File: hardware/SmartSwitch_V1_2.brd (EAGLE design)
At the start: 49 x 49 mm, 47 parts, among them K1 FTR-LYC5, K2 FTR-LYC5, U2 AMS1117-3.3

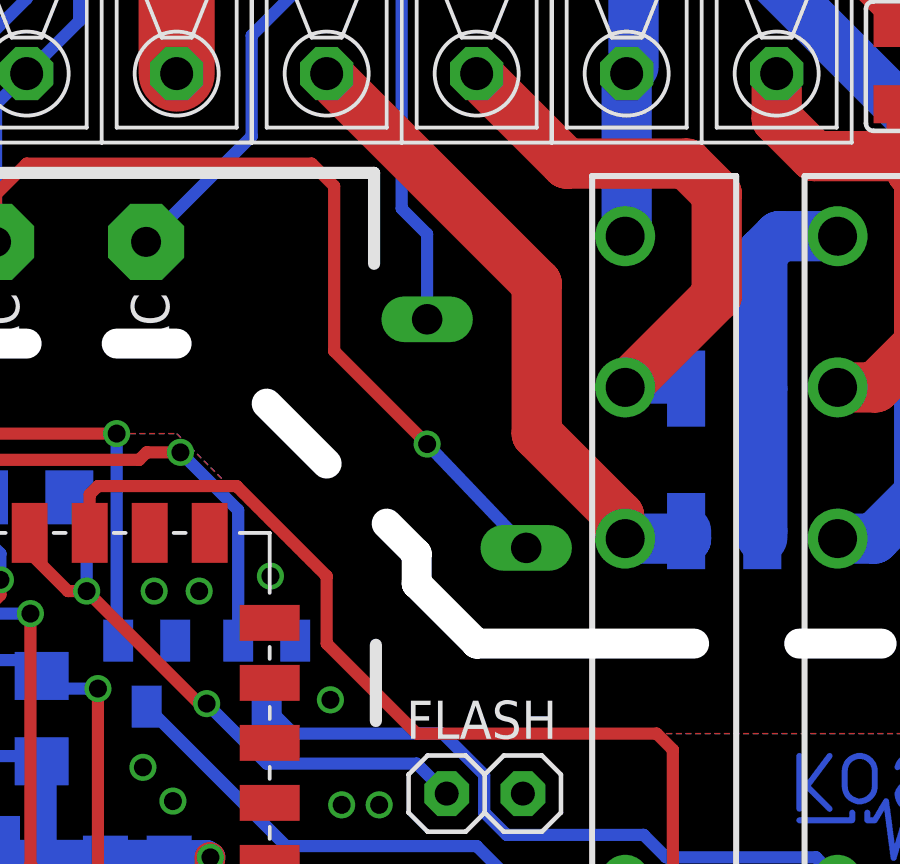
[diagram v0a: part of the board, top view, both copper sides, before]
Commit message: Add files via upload
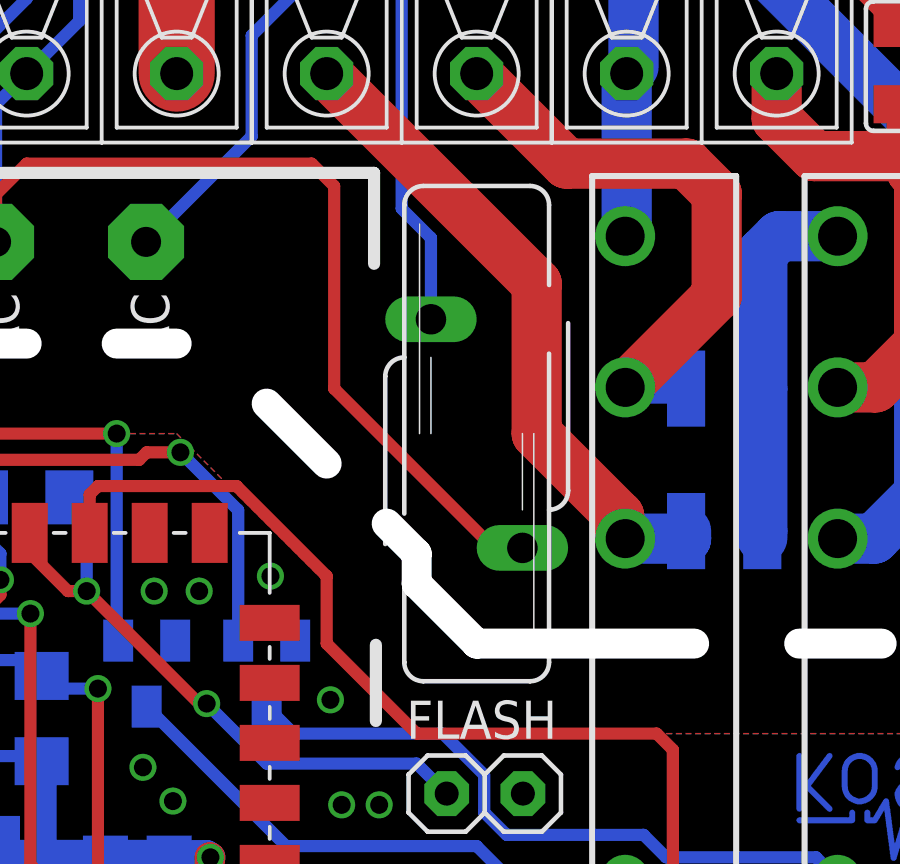
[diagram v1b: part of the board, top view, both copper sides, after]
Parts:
- R7: value S14K275 -> S14K275GESPIEGELT; device varistor:S14K275 -> varistor:S14K275_
- flipped R7 to the top
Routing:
- net HV.N: track 49.5 -> 50.1 mm, vias 1 -> 0
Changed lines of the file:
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@@
 <layer number="23" name="tOrigins" color="15" fill="1" visible="yes" active="yes"/>
 <layer number="24" name="bOrigins" color="15" fill="1" visible="yes" active="yes"/>
-<layer number="25" name="tNames" color="7" fill="1" visible="yes" active="yes"/>
-<layer number="26" name="bNames" color="7" fill="1" visible="yes" active="yes"/>
-<layer number="27" name="tValues" color="7" fill="1" visible="yes" active="yes"/>
-<layer number="28" name="bValues" color="7" fill="1" visible="yes" active="yes"/>
+<layer number="25" name="tNames" color="7" fill="1" visible="no" active="yes"/>
+<layer number="26" name="bNames" color="7" fill="1" visible="no" active="yes"/>
+<layer number="27" name="tValues" color="7" fill="1" visible="no" active="yes"/>
+<layer number="28" name="bValues" color="7" fill="1" visible="no" active="yes"/>
 <layer number="29" name="tStop" color="7" fill="3" visible="no" active="yes"/>
 <layer number="30" name="bStop" color="7" fill="6" visible="no" active="yes"/>
@@
 <attribute name="VALUE" x="17.54" y="19.27" size="1.27" layer="28" rot="MR270"/>
 </element>
-<element name="R7" library="varistor" package="S14K275" value="S14K275" x="32" y="26.5" smashed="yes" rot="MR0">
-<attribute name="VALUE" x="35.429" y="26.119" size="1.27" layer="28" ratio="10" rot="MR90"/>
+<element name="R7" library="varistor" package="S14K275_" value="S14K275GESPIEGELT" x="32" y="26.5" smashed="yes">
+<attribute name="VALUE" x="28.571" y="26.119" size="1.27" layer="27" ratio="10" rot="R90"/>
 </element>
 <element name="F1" library="fuse" package="SMD_FUSE_HOLDER" value="0,4A" x="25" y="43.5" smashed="yes" rot="MR180"/>
@@
 <wire x1="17" y1="35.5" x2="26.5" y2="35.5" width="0.4064" layer="1"/>
 <wire x1="26.5" y1="35.5" x2="27.25" y2="34.75" width="0.4064" layer="1"/>
-<wire x1="27.25" y1="34.75" x2="27.25" y2="29.25" width="0.4064" layer="1"/>
-<wire x1="27.25" y1="29.25" x2="30.349" y2="26.151" width="0.4064" layer="1"/>
-<wire x1="30.349" y1="26.151" x2="33.651" y2="22.69" width="0.4064" layer="16"/>
+<wire x1="27.25" y1="34.75" x2="27.25" y2="28" width="0.4064" layer="1"/>
 <contactref element="R2" pad="1"/>
 <contactref element="R4" pad="1"/>
@@
 <wire x1="18.75" y1="46.25" x2="18.75" y2="40.25" width="0.4064" layer="16"/>
 <wire x1="18.75" y1="40.25" x2="17" y2="38.5" width="0.4064" layer="16"/>
-<via x="30.349" y="26.151" extent="1-16" drill="0.6" shape="octagon"/>
 <wire x1="12.422" y1="46" x2="14.25" y2="46" width="0.4064" layer="16"/>
 <wire x1="14.25" y1="46" x2="14.922" y2="46.672" width="0.4064" layer="16"/>
 <wire x1="14.922" y1="46.672" x2="17" y2="46.672" width="0.4064" layer="16"/>
+<wire x1="27.25" y1="28" x2="32.524" y2="22.726" width="0.4064" layer="1"/>
+<wire x1="32.524" y1="22.726" x2="33.524" y2="22.69" width="0.4064" layer="1"/>
 </signal>
 <signal name="N$8">
@@
 <wire x1="28.19" y1="43.31" x2="28" y2="43.5" width="1" layer="16"/>
 <wire x1="28.19" y1="43.46" x2="28.19" y2="43.31" width="1" layer="16"/>
-<wire x1="29.5" y1="34" x2="30.349" y2="33.151" width="0.4064" layer="16"/>
-<wire x1="30.349" y1="33.151" x2="30.349" y2="30.31" width="0.4064" layer="16"/>
+<wire x1="29.5" y1="34" x2="30.476" y2="33.024" width="0.4064" layer="16"/>
+<wire x1="30.476" y1="33.024" x2="30.476" y2="30.31" width="0.4064" layer="16"/>
 </signal>
 <signal name="RESET">
